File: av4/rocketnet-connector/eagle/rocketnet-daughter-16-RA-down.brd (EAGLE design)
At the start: 19.9 x 7.7 mm, 1 part

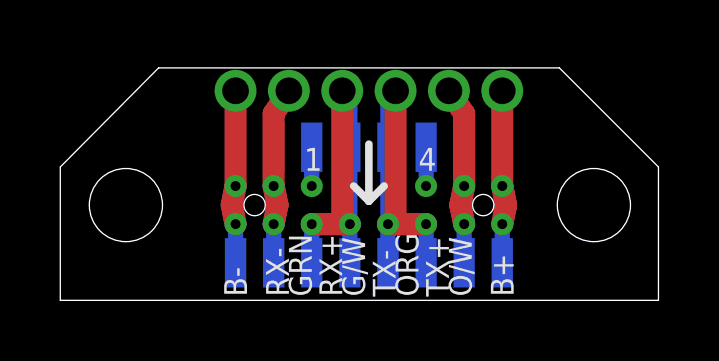
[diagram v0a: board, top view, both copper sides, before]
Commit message: Received boards from OSH Park: made minor changes to board for future runs: moved silk screen and moved edge of board away from wire holes, which are clipped in the first run.
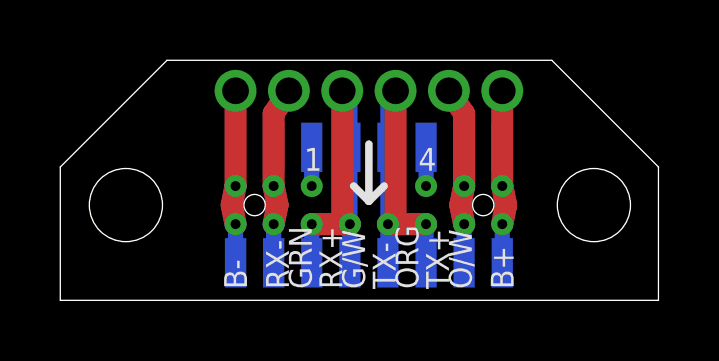
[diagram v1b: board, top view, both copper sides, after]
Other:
- board size 19.9 x 7.7 mm -> 19.9 x 8 mm
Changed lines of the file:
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@@
 <layer number="27" name="tValues" color="7" fill="1" visible="no" active="yes"/>
 <layer number="28" name="bValues" color="7" fill="1" visible="no" active="yes"/>
-<layer number="29" name="tStop" color="7" fill="3" visible="yes" active="yes"/>
+<layer number="29" name="tStop" color="7" fill="3" visible="no" active="yes"/>
 <layer number="30" name="bStop" color="7" fill="6" visible="yes" active="yes"/>
 <layer number="31" name="tCream" color="7" fill="4" visible="no" active="yes"/>
@@
 <plain>
 <wire x1="9.652" y1="-3.175" x2="9.652" y2="1.27" width="0.02" layer="20"/>
-<wire x1="9.652" y1="1.27" x2="6.35" y2="4.572" width="0.02" layer="20"/>
+<wire x1="9.652" y1="1.27" x2="6.096" y2="4.826" width="0.02" layer="20"/>
 <wire x1="9.652" y1="-3.175" x2="-10.287" y2="-3.175" width="0.02" layer="20"/>
 <text x="-3.717" y="5.576" size="0.254" layer="51">TOP VIEW (M50 on bottom of board)</text>
 <hole x="7.5" y="0" drill="2.4384"/>
 <hole x="-8.1" y="0" drill="2.4384"/>
-<wire x1="6.35" y1="4.572" x2="-7.0104" y2="4.572" width="0.02" layer="20"/>
-<wire x1="-7.0104" y1="4.572" x2="-10.287" y2="1.27" width="0.02" layer="20"/>
+<wire x1="6.096" y1="4.826" x2="-6.731" y2="4.826" width="0.02" layer="20"/>
+<wire x1="-6.731" y1="4.826" x2="-10.287" y2="1.27" width="0.02" layer="20"/>
 <wire x1="-10.287" y1="1.27" x2="-10.287" y2="-3.175" width="0.02" layer="20"/>
 <circle x="7.493" y="-0.0762" radius="2.159" width="0.0254" layer="51"/>
@@
 <text x="-2.921" y="-7.493" size="0.254" layer="51">Entire "ribbon": 0.275 in</text>
 <wire x1="9.271" y1="5.08" x2="11.049" y2="5.08" width="0.0254" layer="51"/>
-<text x="4.826" y="-3.048" size="0.762" layer="21" ratio="20" rot="R90">B+</text>
-<text x="-4.064" y="-3.048" size="0.762" layer="21" ratio="20" rot="R90">B-</text>
+<text x="4.826" y="-2.794" size="0.762" layer="21" ratio="20" rot="R90">B+</text>
+<text x="-4.064" y="-2.794" size="0.762" layer="21" ratio="20" rot="R90">B-</text>
 <text x="-2.159" y="1.143" size="0.762" layer="21" ratio="20">1</text>
 <text x="1.651" y="1.143" size="0.762" layer="21" ratio="20">4</text>
@@
 <text x="8.763" y="-2.54" size="0.762" layer="22" ratio="20" rot="MR0">PSAS</text>
 <text x="11.176" y="4.445" size="0.254" layer="51">Edge of RNH PCB</text>
-<text x="-2.667" y="-3.048" size="0.762" layer="21" ratio="20" rot="R90">RX-</text>
-<text x="-0.889" y="-3.048" size="0.762" layer="21" ratio="20" rot="R90">RX+</text>
-<text x="0.889" y="-3.048" size="0.762" layer="21" ratio="20" rot="R90">TX-</text>
-<text x="2.667" y="-3.048" size="0.762" layer="21" ratio="20" rot="R90">TX+</text>
+<text x="-2.667" y="-2.794" size="0.762" layer="21" ratio="20" rot="R90">RX-</text>
+<text x="-0.889" y="-2.794" size="0.762" layer="21" ratio="20" rot="R90">RX+</text>
+<text x="0.889" y="-2.794" size="0.762" layer="21" ratio="20" rot="R90">TX-</text>
+<text x="2.667" y="-2.794" size="0.762" layer="21" ratio="20" rot="R90">TX+</text>
 <text x="-6.477" y="-2.54" size="0.762" layer="22" ratio="20" rot="MR0">RNCv1</text>
 <text x="11.176" y="4.953" size="0.254" layer="51">Edge of top plate</text>
@@
 <wire x1="10.287" y1="1.905" x2="10.795" y2="2.413" width="0.0254" layer="51"/>
 <text x="10.922" y="2.286" size="0.254" layer="51">Tool OD</text>
-<text x="3.429" y="-3.048" size="0.762" layer="21" ratio="20" rot="R90">O/W</text>
-<text x="1.651" y="-3.048" size="0.762" layer="21" ratio="20" rot="R90">ORG</text>
-<text x="-0.127" y="-3.048" size="0.762" layer="21" ratio="20" rot="R90">G/W</text>
-<text x="-1.905" y="-3.048" size="0.762" layer="21" ratio="20" rot="R90">GRN</text>
+<text x="3.429" y="-2.794" size="0.762" layer="21" ratio="20" rot="R90">O/W</text>
+<text x="1.651" y="-2.794" size="0.762" layer="21" ratio="20" rot="R90">ORG</text>
+<text x="-0.127" y="-2.794" size="0.762" layer="21" ratio="20" rot="R90">G/W</text>
+<text x="-1.905" y="-2.794" size="0.762" layer="21" ratio="20" rot="R90">GRN</text>
 <wire x1="9.3218" y1="4.5466" x2="11.0998" y2="4.5466" width="0.0254" layer="51"/>
+<circle x="-1.905" y="0.635" radius="0.381" width="0" layer="29"/>
+<circle x="1.905" y="0.635" radius="0.381" width="0" layer="29"/>
+<circle x="1.905" y="0.635" radius="0.381" width="0" layer="30"/>
+<circle x="-1.905" y="0.635" radius="0.381" width="0" layer="30"/>
 </plain>
 <attributes>
